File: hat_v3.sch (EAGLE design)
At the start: 37 parts, among them U1 ADS1115IDGST, U2 ADXL345, U5 MCP2515-I/ST, U6 MCP2551

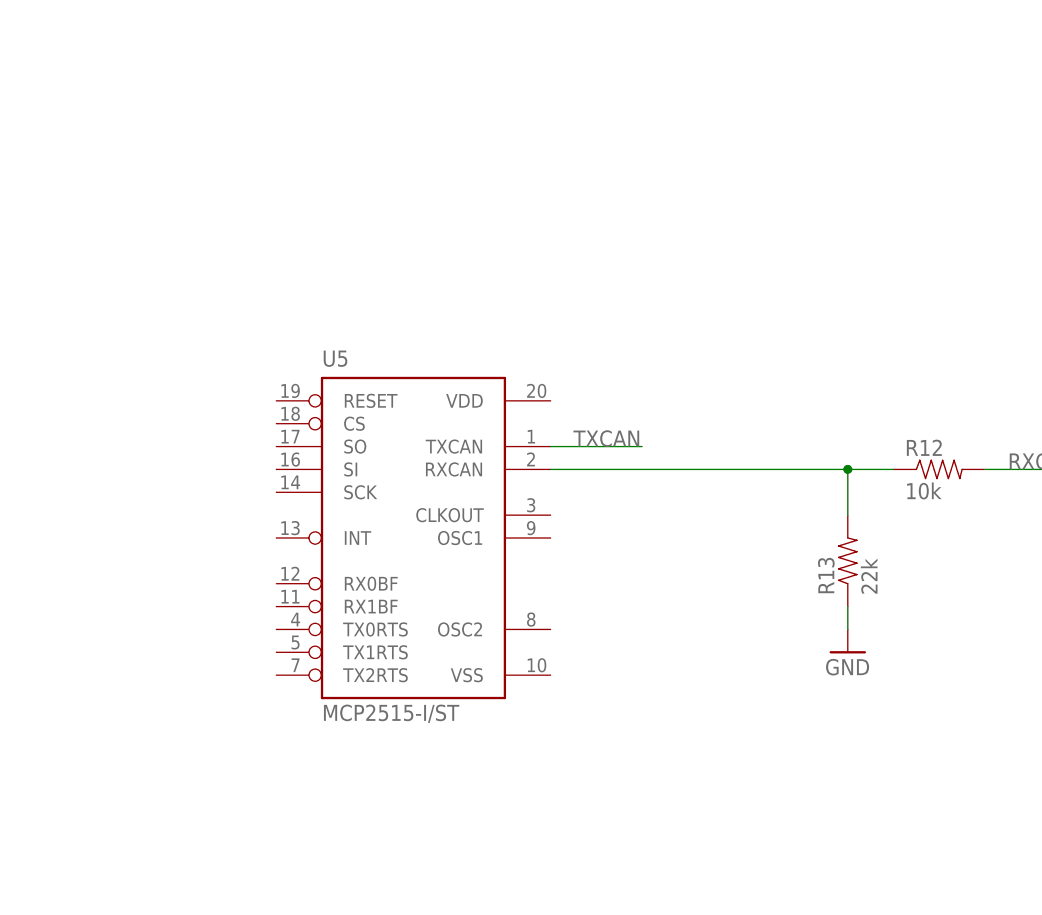
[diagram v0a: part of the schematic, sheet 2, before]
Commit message: V3 done!
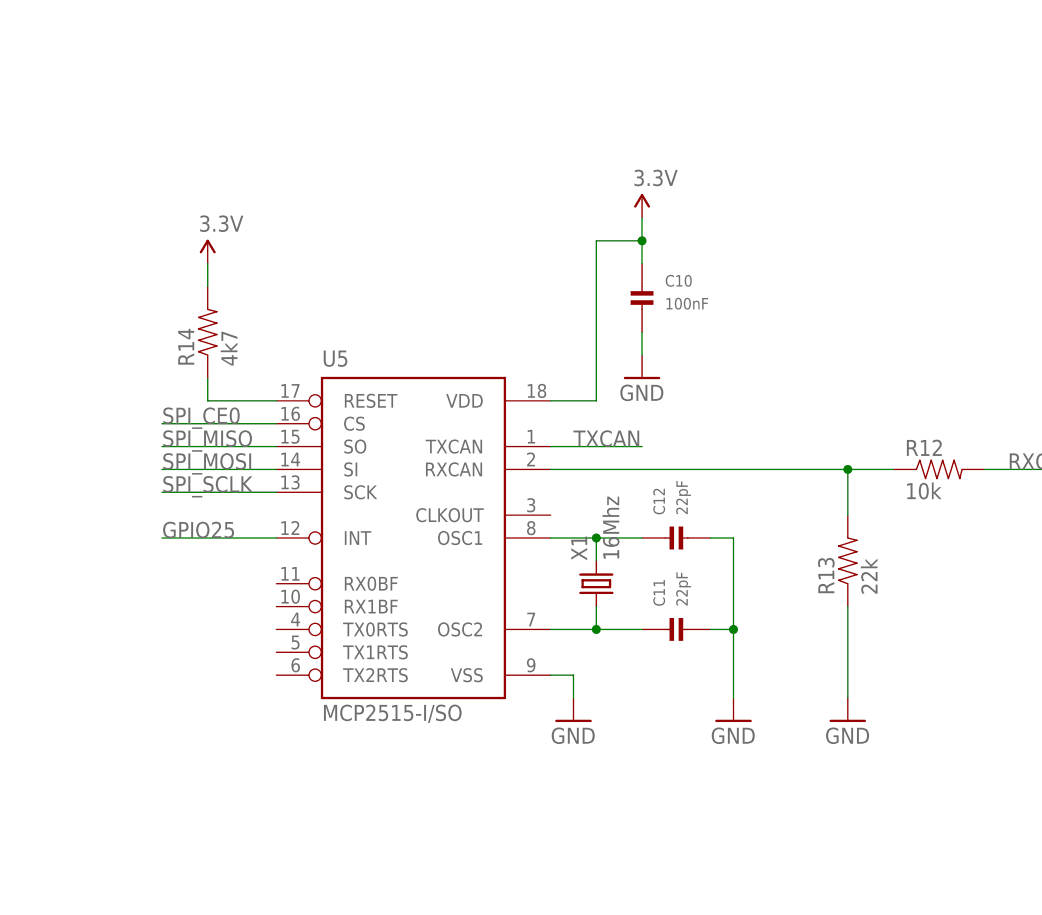
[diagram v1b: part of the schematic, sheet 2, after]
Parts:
- added C10: 100nF, microbuilder:CAP_CERAMIC0805
- added C11, C12: 22pF, microbuilder:CAP_CERAMIC0805
- added R14: 4k7, SparkFun-Passives:RESISTOR0805-RES
- added X1: 16Mhz, IQD-Frequency-Products:CRYSTALS-NOGND-4-HSMX
- U5: value MCP2515-I/ST -> MCP2515-I/SO; device mcp2515:MCP2515-I/ST -> mcp2515:MCP2515-I/SO
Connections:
- new net N$14: C12.P$1, U5.OSC1, X1.2
- new net N$15: C11.P$1, U5.OSC2, X1.1
- new net U5_RST: R14.1, U5.RESET
- net 3.3V: now also C10.P$1, R14.2, U5.VDD
- net GND: now also C10.P$2, C11.P$2, C12.P$2, U5.VSS
- net GPIO25: now also U5.INT
- net SPI_CE0: now also U5.CS
- net SPI_MISO: now also U5.SO
- net SPI_MOSI: now also U5.SI
- net SPI_SCLK: now also U5.SCK
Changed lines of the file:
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@@
 <part name="D1" library="diode" deviceset="DIODE-" device="DO214AC"/>
 <part name="SUPPLY9" library="SparkFun-Aesthetics" deviceset="5V" device=""/>
-<part name="U5" library="mcp2515" deviceset="MCP2515" device="-I/ST"/>
 <part name="U6" library="SparkFun-DigitalIC" deviceset="MCP2551" device=""/>
 <part name="R9" library="SparkFun-Passives" deviceset="RESISTOR" device="0805-RES" value="4k7"/>
@@
 <part name="R13" library="SparkFun-Passives" deviceset="RESISTOR" device="0805-RES" value="22k"/>
 <part name="GND6" library="SparkFun-Aesthetics" deviceset="GND" device=""/>
+<part name="SUPPLY10" library="SparkFun-Aesthetics" deviceset="3.3V" device=""/>
+<part name="R14" library="SparkFun-Passives" deviceset="RESISTOR" device="0805-RES" value="4k7"/>
+<part name="SUPPLY12" library="SparkFun-Aesthetics" deviceset="3.3V" device=""/>
+<part name="C10" library="microbuilder" deviceset="CAP_CERAMIC" device="0805" value="100nF"/>
+<part name="GND8" library="SparkFun-Aesthetics" deviceset="GND" device=""/>
+<part name="GND9" library="SparkFun-Aesthetics" deviceset="GND" device=""/>
+<part name="X1" library="IQD-Frequency-Products" deviceset="CRYSTALS-NOGND" device="-4-HSMX" value="16Mhz"/>
+<part name="C11" library="microbuilder" deviceset="CAP_CERAMIC" device="0805" value="22pF"/>
+<part name="C12" library="microbuilder" deviceset="CAP_CERAMIC" device="0805" value="22pF"/>
+<part name="GND10" library="SparkFun-Aesthetics" deviceset="GND" device=""/>
+<part name="U5" library="mcp2515" deviceset="MCP2515" device="-I/SO"/>
 </parts>
 <sheets>
@@
 </plain>
 <instances>
-<instance part="U5" gate="G$1" x="58.42" y="99.06"/>
 <instance part="U6" gate="MCP2551" x="53.34" y="38.1"/>
 <instance part="R9" gate="G$1" x="83.82" y="27.94" rot="R90"/>
@@
 <instance part="R12" gate="G$1" x="116.84" y="106.68"/>
 <instance part="R13" gate="G$1" x="106.68" y="96.52" rot="R90"/>
-<instance part="GND6" gate="1" x="106.68" y="86.36"/>
+<instance part="GND6" gate="1" x="106.68" y="78.74"/>
+<instance part="SUPPLY10" gate="G$1" x="35.56" y="129.54"/>
+<instance part="R14" gate="G$1" x="35.56" y="121.92" rot="R90"/>
+<instance part="SUPPLY12" gate="G$1" x="83.82" y="134.62"/>
+<instance part="C10" gate="G$1" x="83.82" y="124.46"/>
+<instance part="GND8" gate="1" x="83.82" y="116.84"/>
+<instance part="GND9" gate="1" x="76.2" y="78.74"/>
+<instance part="X1" gate="G$1" x="78.74" y="93.98" rot="R90"/>
+<instance part="C11" gate="G$1" x="88.9" y="88.9" rot="R90"/>
+<instance part="C12" gate="G$1" x="88.9" y="99.06" rot="R90"/>
+<instance part="GND10" gate="1" x="93.98" y="78.74"/>
+<instance part="U5" gate="G$1" x="58.42" y="99.06"/>
 </instances>
 <busses>
@@
 <pinref part="R13" gate="G$1" pin="1"/>
 <pinref part="GND6" gate="1" pin="GND"/>
-<wire x1="106.68" y1="91.44" x2="106.68" y2="88.9" width="0.1524" layer="91"/>
+<wire x1="106.68" y1="91.44" x2="106.68" y2="81.28" width="0.1524" layer="91"/>
+</segment>
+<segment>
+<pinref part="GND8" gate="1" pin="GND"/>
+<pinref part="C10" gate="G$1" pin="P$2"/>
+<wire x1="83.82" y1="119.38" x2="83.82" y2="121.92" width="0.1524" layer="91"/>
+</segment>
+<segment>
+<pinref part="GND9" gate="1" pin="GND"/>
+<wire x1="73.66" y1="83.82" x2="76.2" y2="83.82" width="0.1524" layer="91"/>
+<wire x1="76.2" y1="83.82" x2="76.2" y2="81.28" width="0.1524" layer="91"/>
+<pinref part="U5" gate="G$1" pin="VSS"/>
+</segment>
+<segment>
+<pinref part="C11" gate="G$1" pin="P$2"/>
+<wire x1="91.44" y1="88.9" x2="93.98" y2="88.9" width="0.1524" layer="91"/>
+<wire x1="93.98" y1="88.9" x2="93.98" y2="81.28" width="0.1524" layer="91"/>
+<pinref part="C12" gate="G$1" pin="P$2"/>
+<wire x1="91.44" y1="99.06" x2="93.98" y2="99.06" width="0.1524" layer="91"/>
+<wire x1="93.98" y1="99.06" x2="93.98" y2="88.9" width="0.1524" layer="91"/>
+<pinref part="GND10" gate="1" pin="GND"/>
+<junction x="93.98" y="88.9"/>
 </segment>
 </net>
@@
 </segment>
 <segment>
-<pinref part="U5" gate="G$1" pin="TXCAN"/>
 <wire x1="73.66" y1="109.22" x2="83.82" y2="109.22" width="0.1524" layer="91"/>
 <label x="76.2" y="109.22" size="1.778" layer="95"/>
+<pinref part="U5" gate="G$1" pin="TXCAN"/>
 </segment>
 </net>
@@
 <segment>
 <pinref part="R12" gate="G$1" pin="1"/>
-<pinref part="U5" gate="G$1" pin="RXCAN"/>
 <wire x1="111.76" y1="106.68" x2="106.68" y2="106.68" width="0.1524" layer="91"/>
 <pinref part="R13" gate="G$1" pin="2"/>
@@
 <wire x1="106.68" y1="101.6" x2="106.68" y2="106.68" width="0.1524" layer="91"/>
 <junction x="106.68" y="106.68"/>
+<pinref part="U5" gate="G$1" pin="RXCAN"/>
+</segment>
+</net>
+<net name="3.3V" class="0">
+<segment>
+<wire x1="35.56" y1="127" x2="35.56" y2="129.54" width="0.1524" layer="91"/>
+<pinref part="SUPPLY10" gate="G$1" pin="3.3V"/>
+<pinref part="R14" gate="G$1" pin="2"/>
+</segment>
+<segment>
+<pinref part="C10" gate="G$1" pin="P$1"/>
+<pinref part="SUPPLY12" gate="G$1" pin="3.3V"/>
+<wire x1="83.82" y1="129.54" x2="83.82" y2="132.08" width="0.1524" layer="91"/>
+<wire x1="83.82" y1="132.08" x2="83.82" y2="134.62" width="0.1524" layer="91"/>
+<wire x1="73.66" y1="114.3" x2="78.74" y2="114.3" width="0.1524" layer="91"/>
+<wire x1="78.74" y1="114.3" x2="78.74" y2="132.08" width="0.1524" layer="91"/>
+<wire x1="78.74" y1="132.08" x2="83.82" y2="132.08" width="0.1524" layer="91"/>
+<junction x="83.82" y="132.08"/>
+<pinref part="U5" gate="G$1" pin="VDD"/>
+</segment>
+</net>
+<net name="U5_RST" class="0">
+<segment>
+<wire x1="43.18" y1="114.3" x2="35.56" y2="114.3" width="0.1524" layer="91"/>
+<wire x1="35.56" y1="114.3" x2="35.56" y2="116.84" width="0.1524" layer="91"/>
+<pinref part="R14" gate="G$1" pin="1"/>
+<pinref part="U5" gate="G$1" pin="RESET"/>
+</segment>
+</net>
+<net name="SPI_CE0" class="0">
+<segment>
+<wire x1="43.18" y1="111.76" x2="30.48" y2="111.76" width="0.1524" layer="91"/>
+<label x="30.48" y="111.76" size="1.778" layer="95"/>
+<pinref part="U5" gate="G$1" pin="CS"/>
+</segment>
+</net>
+<net name="SPI_SCLK" class="0">
+<segment>
+<wire x1="43.18" y1="104.14" x2="30.48" y2="104.14" width="0.1524" layer="91"/>
+<label x="30.48" y="104.14" size="1.778" layer="95"/>
+<pinref part="U5" gate="G$1" pin="SCK"/>
+</segment>
+</net>
+<net name="GPIO25" class="0">
+<segment>
+<wire x1="43.18" y1="99.06" x2="30.48" y2="99.06" width="0.1524" layer="91"/>
+<label x="30.48" y="99.06" size="1.778" layer="95"/>
+<pinref part="U5" gate="G$1" pin="INT"/>
+</segment>
+</net>
+<net name="N$14" class="0">
+<segment>
+<wire x1="73.66" y1="99.06" x2="78.74" y2="99.06" width="0.1524" layer="91"/>
+<pinref part="X1" gate="G$1" pin="2"/>
+<wire x1="78.74" y1="99.06" x2="78.74" y2="96.52" width="0.1524" layer="91"/>
+<pinref part="C12" gate="G$1" pin="P$1"/>
+<wire x1="78.74" y1="99.06" x2="83.82" y2="99.06" width="0.1524" layer="91"/>
+<junction x="78.74" y="99.06"/>
+<pinref part="U5" gate="G$1" pin="OSC1"/>
+</segment>
+</net>
+<net name="N$15" class="0">
+<segment>
+<wire x1="73.66" y1="88.9" x2="78.74" y2="88.9" width="0.1524" layer="91"/>
+<pinref part="X1" gate="G$1" pin="1"/>
+<wire x1="78.74" y1="88.9" x2="78.74" y2="91.44" width="0.1524" layer="91"/>
+<pinref part="C11" gate="G$1" pin="P$1"/>
+<wire x1="83.82" y1="88.9" x2="78.74" y2="88.9" width="0.1524" layer="91"/>
+<junction x="78.74" y="88.9"/>
+<pinref part="U5" gate="G$1" pin="OSC2"/>
+</segment>
+</net>
+<net name="SPI_MISO" class="0">
+<segment>
+<wire x1="43.18" y1="109.22" x2="30.48" y2="109.22" width="0.1524" layer="91"/>
+<label x="30.48" y="109.22" size="1.778" layer="95"/>
+<pinref part="U5" gate="G$1" pin="SO"/>
+</segment>
+</net>
+<net name="SPI_MOSI" class="0">
+<segment>
+<wire x1="43.18" y1="106.68" x2="30.48" y2="106.68" width="0.1524" layer="91"/>
+<label x="30.48" y="106.68" size="1.778" layer="95"/>
+<pinref part="U5" gate="G$1" pin="SI"/>
 </segment>
 </net>
@@
 </sheet>
 </sheets>
+<errors>
+</errors>
 </schematic>
 </drawing>
